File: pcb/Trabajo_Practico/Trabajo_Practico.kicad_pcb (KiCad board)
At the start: 2 copper layers, 71.6 x 60.5 mm, 17 parts, among them J1 Conn_02x19_Odd_Even, J2 Conn_02x19_Odd_Even, J3 Conn_01x03_Male, J4 Conn_01x03_Male, J5 SD_Card_P, U1 ESP8266-01_ESP-01, U2 MAX30102_P, U4 DS18B20

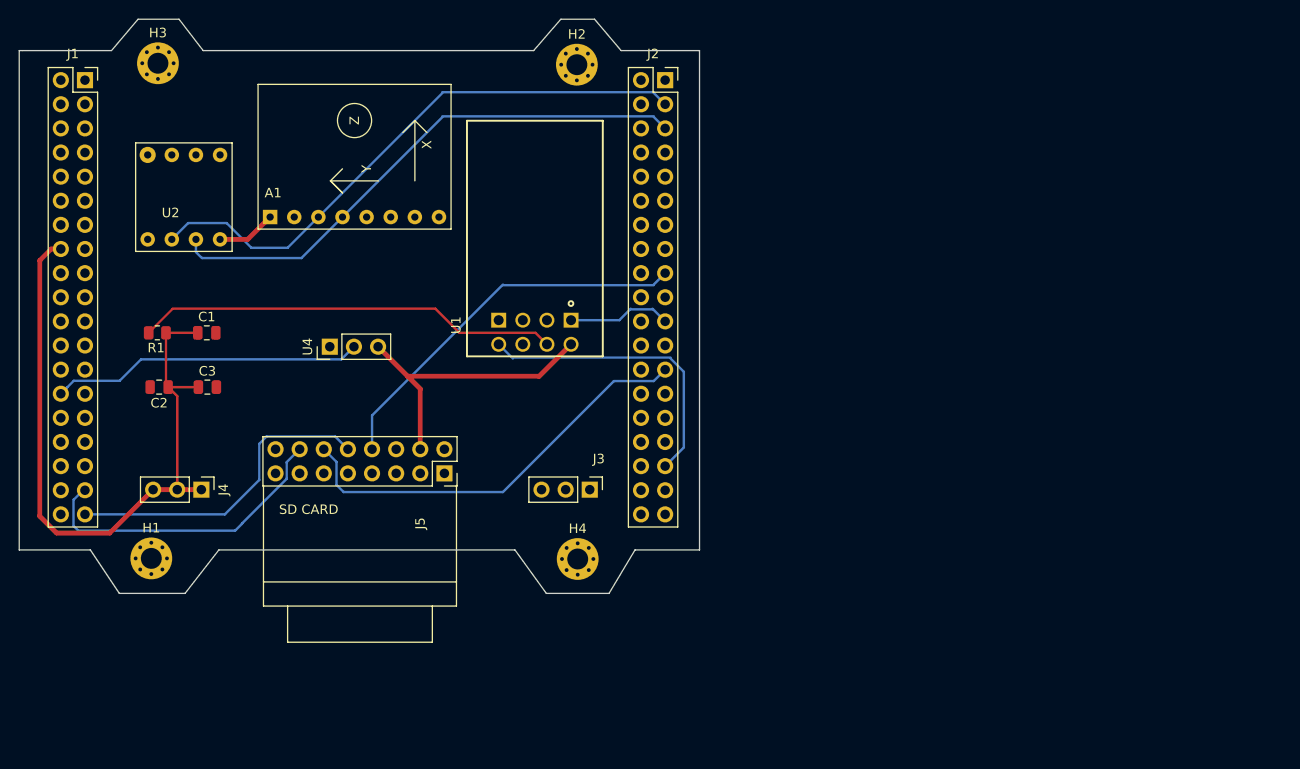
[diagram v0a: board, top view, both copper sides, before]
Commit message: Presentacion final del proyecto
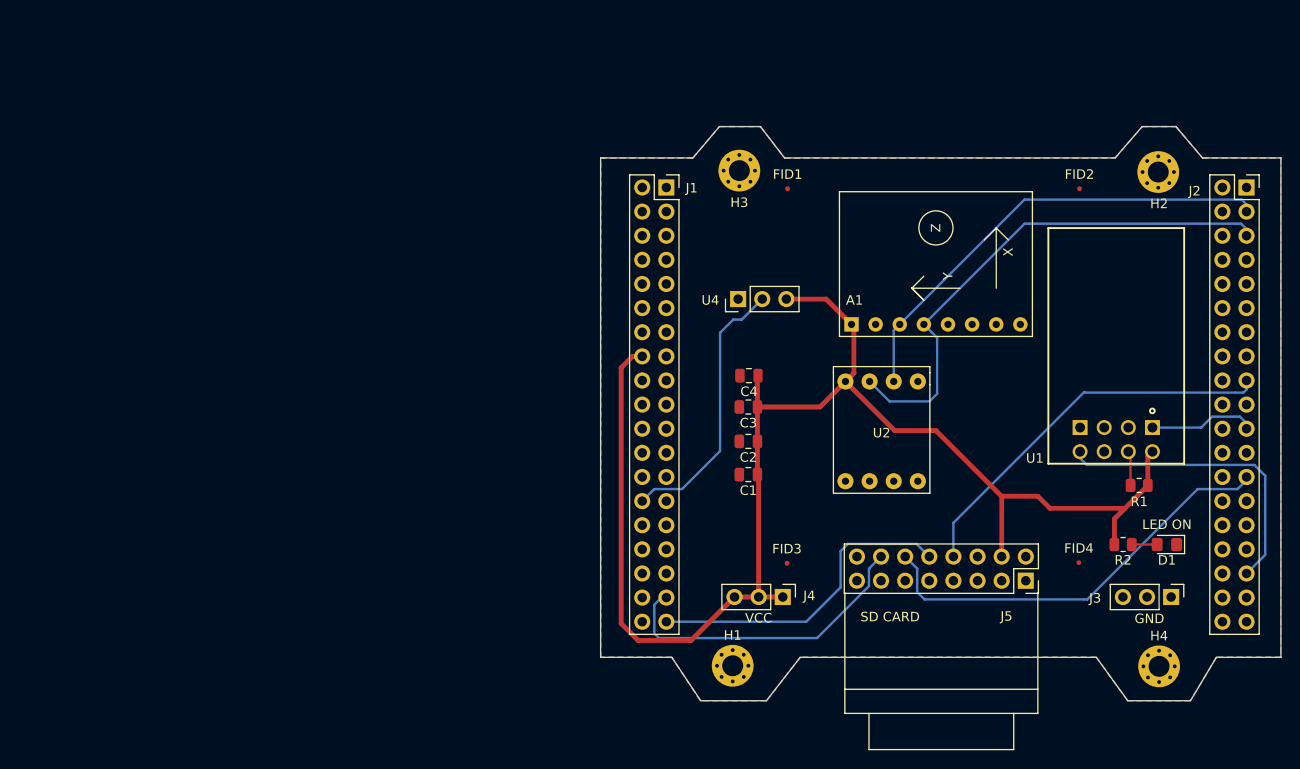
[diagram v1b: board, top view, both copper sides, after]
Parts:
- added C4: 100nF, Capacitor_SMD:C_0805_2012Metric, F.Cu at (116.3, 83.2)
- added D1: LED, LED_SMD:LED_0805_2012Metric_Pad1.15x1.40mm_HandSolder, F.Cu at (160.3, 101.0)
- added FID1: Fiducial, Fiducial:Fiducial_0.5mm_Mask1mm, F.Cu at (120.4, 63.6)
- added FID2: Fiducial, Fiducial:Fiducial_0.5mm_Mask1mm, F.Cu at (151.1, 63.6)
- added FID3: Fiducial, Fiducial:Fiducial_0.5mm_Mask1mm, F.Cu at (120.3, 103.0)
- added FID4: Fiducial, Fiducial:Fiducial_0.5mm_Mask1mm, F.Cu at (151.1, 102.9)
- added R2: 330, Resistor_SMD:R_0805_2012Metric, F.Cu at (155.7, 101.0)
- moved R1 104.6 mm to (157.4, 94.8)
- moved U2 83.4 mm to (131.6, 94.4), turned to 180 degrees
- moved C2 62.3 mm to (116.3, 90.2)
- moved H2 62.2 mm to (159.4, 61.8)
- moved J2 62.2 mm to (168.7, 63.4)
- moved J3 62.2 mm to (160.8, 106.6)
- moved H1 62.2 mm to (114.6, 113.8)
- moved H3 62.2 mm to (115.3, 61.7)
- moved J4 62.2 mm to (119.9, 106.6)
- moved A1 62.2 mm to (127.1, 77.9)
- moved H4 62.2 mm to (159.5, 113.9)
- moved J5 62.2 mm to (145.5, 104.8)
- moved U1 62.2 mm to (155.0, 88.7)
- moved J1 62.2 mm to (107.6, 63.4)
- moved C1 58.9 mm to (116.3, 93.7), turned to 180 degrees
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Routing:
- net Net-(R1-Pad1): track 44.5 -> 3.65 mm
- net VCC: track 110.6 -> 151.1 mm
- net /PB8: track 61.0 -> 49.2 mm
- net /AN0: track 32.9 -> 28.7 mm
- net Net-(D1-Pad2): track 0.00 -> 2.67 mm
- net /PB9: track 57.6 -> 55.5 mm
- net /PA10: track 31.4 -> 32.1 mm
- net /CS: track 40.6 -> 41.2 mm
- net /MISO: track 33.0 -> 33.5 mm
- added copper zone on B.Cu, net GND
- added copper zone on F.Cu, net GND
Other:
- board text added: "16/08/21"
- board text added: "GND"
- board text added: "Ing. William's Limonchi FIUBA"
- board text added: "LED ON"
- board text added: "LIMA - PERÚ"
- board text added: "Módulo Detector de Caídas para núcelo STM32 v1.0"
- board text added: "Tamaño de placa * 72 mm * 61 mm Grilla: * 1 mm * 0.25 mm posicionamiento de componentes Tamaños: * 0.25 y 0.5 mm ancho de pista * 0.8 mm pad de vía * 0.5 mm agujero de vía Capas: Top: F.Cu Bottom: B.Cu"
- board text added: "VCC"
